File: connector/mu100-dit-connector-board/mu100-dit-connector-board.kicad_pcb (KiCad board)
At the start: 2 copper layers, 37 x 13.9 mm, 8 parts, among them J1 Conn_01x17_Male, J2 Conn_01x17, J3 Conn_01x10_Female

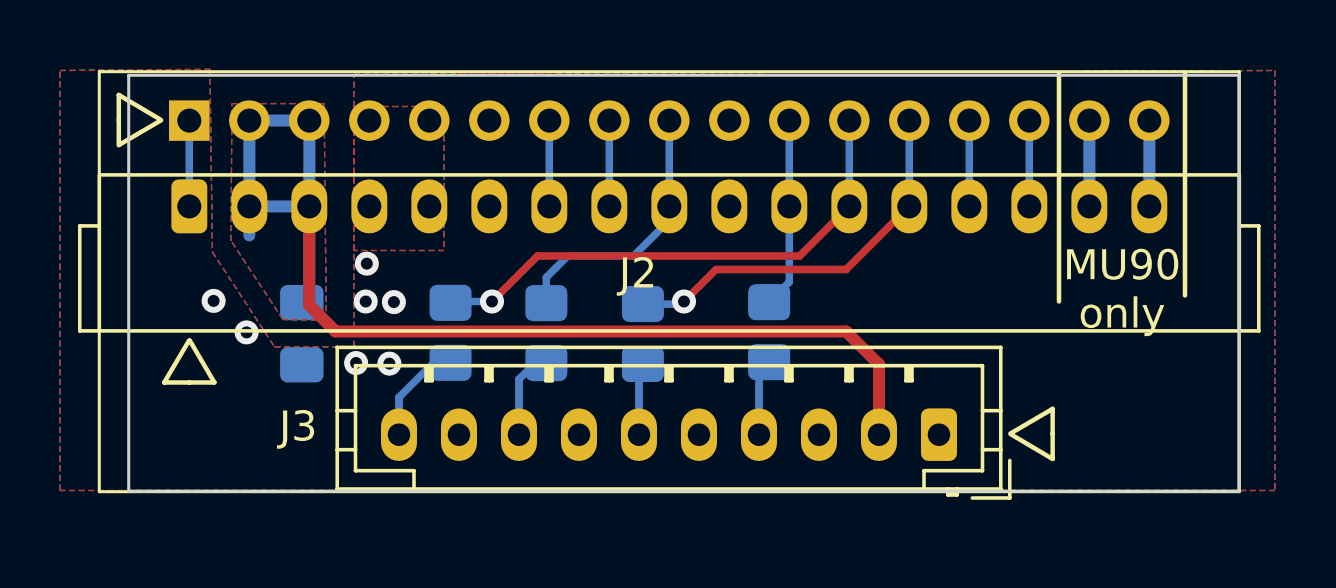
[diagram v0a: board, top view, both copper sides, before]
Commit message: finish connector pcb
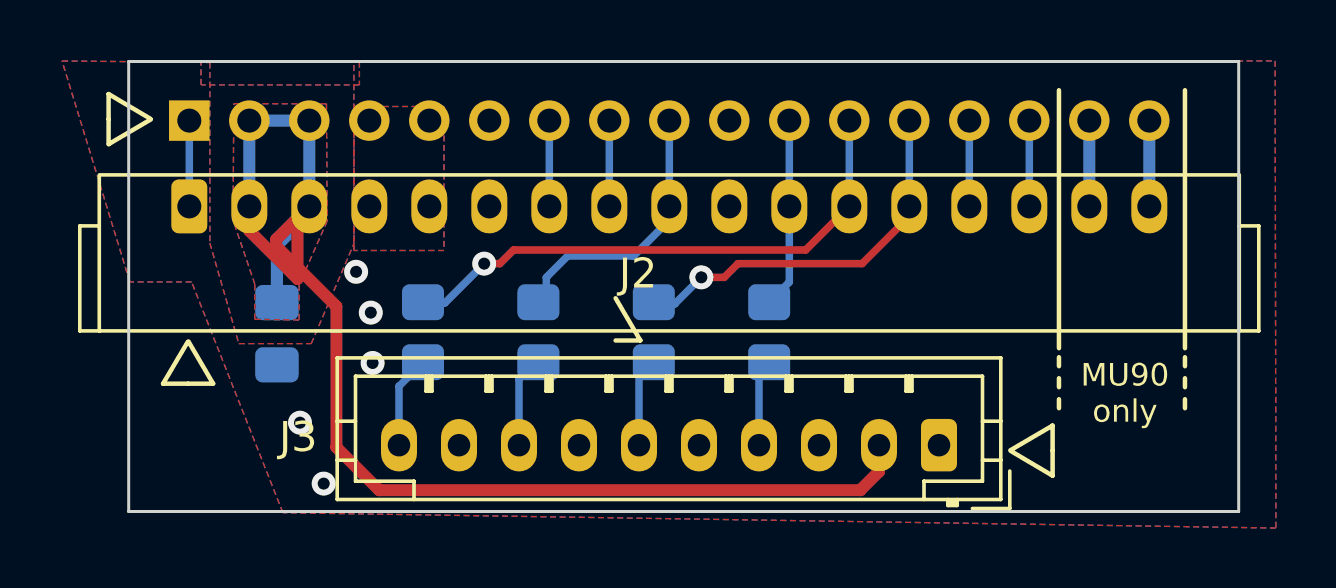
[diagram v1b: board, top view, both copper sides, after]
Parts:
- moved R4 0.92 mm to (73.5, 65.0)
- moved C1 0.83 mm to (68.6, 65.1)
- moved R3 0.37 mm to (81.2, 65.0)
- moved J3 0.35 mm to (90.7, 68.8)
- moved R2 0.27 mm to (77.3, 65.0)
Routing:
- net +5V: track 39.1 -> 49.3 mm
- net /WCLK: track 17.5 -> 18.4 mm
- net /LRCK: track 3.60 -> 2.94 mm
- net GND: track 0.00 -> 0.26 mm, vias 7 -> 5
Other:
- board size 37 x 13.9 mm -> 37 x 15 mm
- board text added: "+9VA"
- board text added: "100"
- board text added: "47"
- board text added: "5V"
- board text added: "AGND"
- board text added: "CK256 (MCLK)"
- board text added: "DACOL (SDAT)"
- board text added: "MELO0"
- board text added: "Molex connector on board"
- board text added: "QCLK (BCK)"
- board text added: "REA"
- board text added: "REB"
- board text added: "RER"
- board text added: "SYOD"
- board text added: "WCLK (LRCK)"
- board text added: "github.com/ nikitalita/ MU100-DIT"

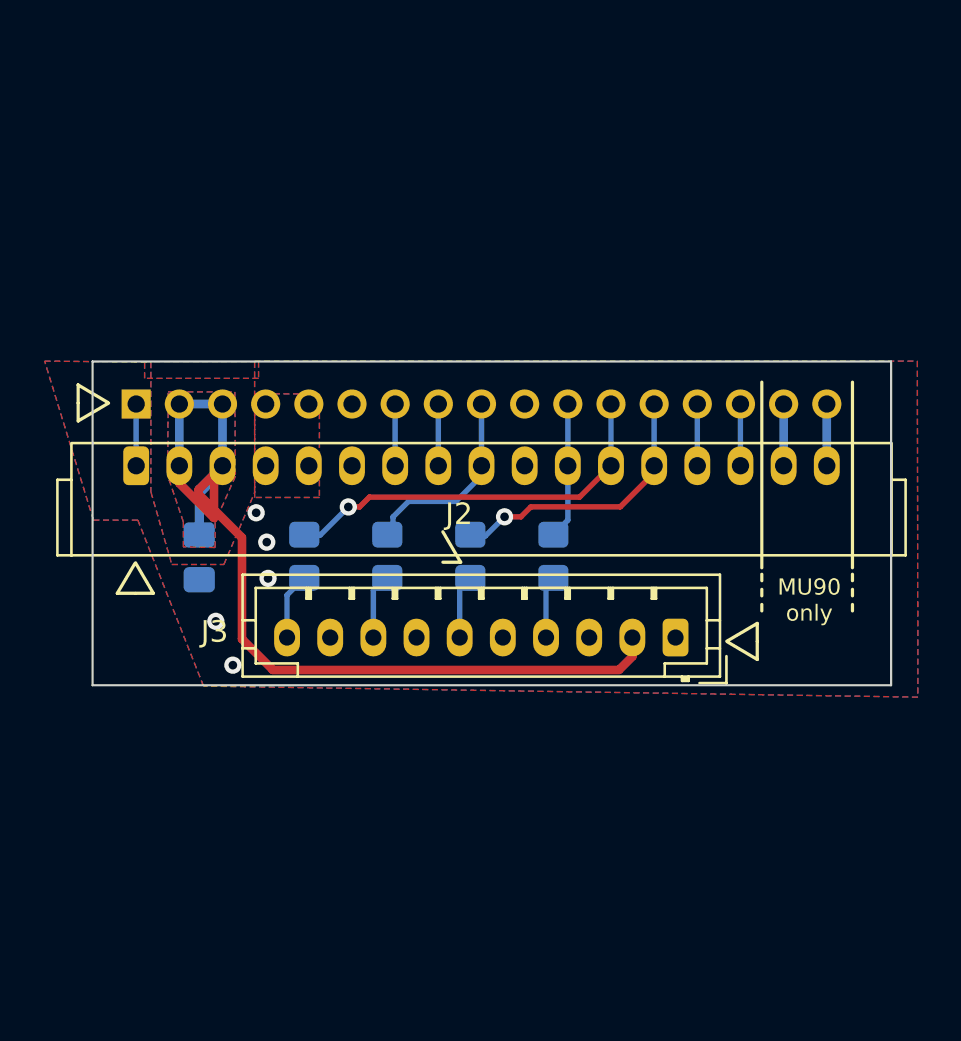
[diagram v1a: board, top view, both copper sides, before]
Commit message: combine pcb projects
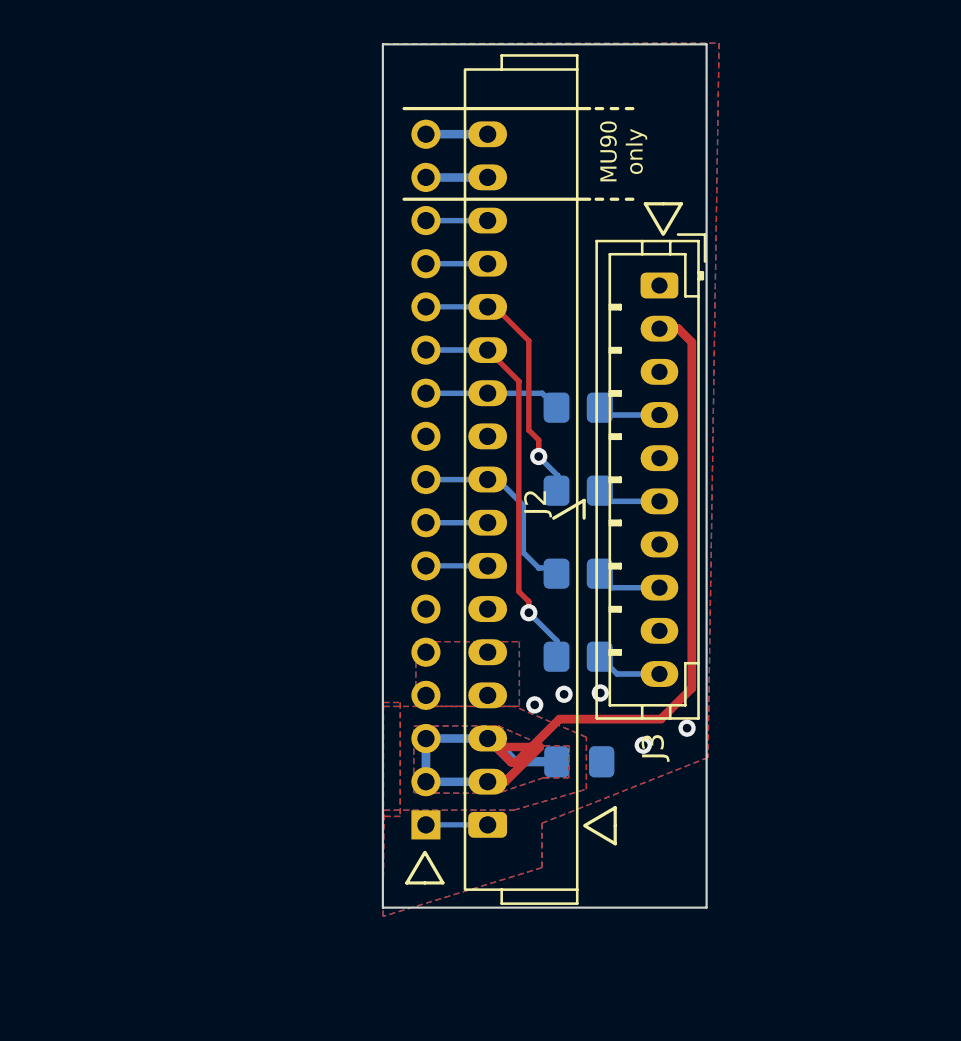
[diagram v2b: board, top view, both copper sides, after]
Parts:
- moved J1 23.7 mm to (79.1, 77.5), turned to 0 degrees
- moved J2 23.3 mm to (82.0, 77.5), turned to 90 degrees
- moved C1 20.0 mm to (86.2, 74.5), turned to 0 degrees
- moved J3 16.3 mm to (90.0, 52.5), turned to -90 degrees
- moved R4 13.5 mm to (86.2, 69.7), turned to 0 degrees
- moved R2 8.88 mm to (86.2, 65.8), turned to 0 degrees
- moved R1 6.98 mm to (86.2, 58.1), turned to 0 degrees
- moved R3 5.85 mm to (86.2, 62.0), turned to 0 degrees
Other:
- board size 37 x 15 mm -> 15 x 40 mm

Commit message: WIP
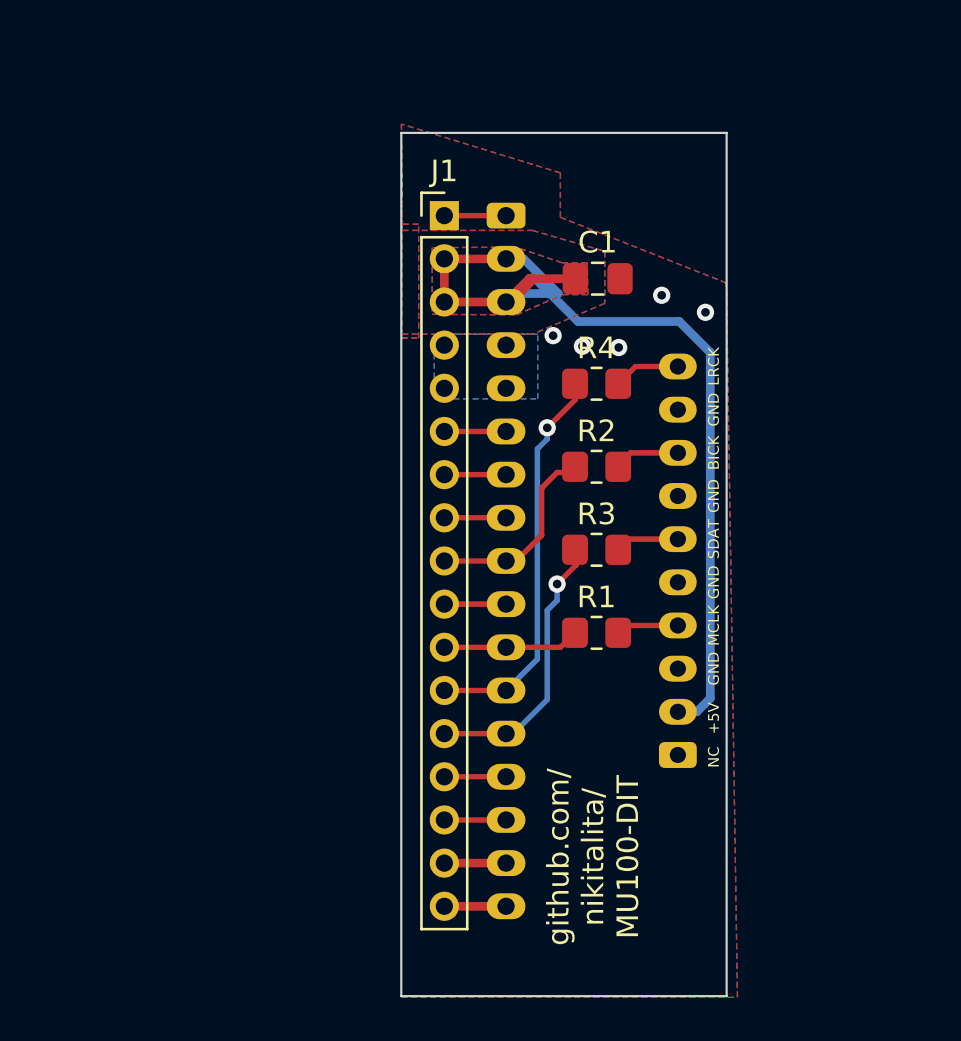
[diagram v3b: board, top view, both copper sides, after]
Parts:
- C1, J1, R1, R2, R3, R4: moved to F.Cu
- J2: value Conn_01x17 -> 51247 Molex; moved to B.Cu
- J3: value Conn_01x10_Female -> JST-PH_01x10_Socket; moved to B.Cu
- moved J1 28.2 mm to (80.0, 49.2)
- moved J2 28.2 mm to (82.8, 49.2), turned to -90 degrees
- moved C1 22.4 mm to (87.1, 52.2)
- moved J3 21.8 mm to (90.8, 74.2), turned to 90 degrees
- moved R4 12.7 mm to (87.0, 57.0)
- moved R1 10.5 mm to (87.0, 68.6)
- moved R2 5.03 mm to (87.0, 60.9)
- moved R3 2.87 mm to (87.0, 64.7)
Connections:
- J1 pad 10: unconnected-(J1-Pad10) -> Net-(J1-Pad10)
- J1 pad 6: unconnected-(J1-Pad6) -> Net-(J1-Pad6)
- J2 pad 10: unconnected-(J2-Pad10) -> Net-(J1-Pad10)
- J2 pad 6: unconnected-(J2-Pad6) -> Net-(J1-Pad6)
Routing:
- net Net-(J1-Pad6): track 0.00 -> 2.86 mm
- net Net-(J1-Pad10): track 0.00 -> 2.86 mm
- net +5V: track 49.3 -> 46.8 mm
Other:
- board size 15 x 40 mm -> 15.1 x 40 mm
- board text added: "16-17 MU90 only"
- board text added: "MU90/100R: Slots into Molex connector MU90/100: Soldered onto unpopulated header"
- board text removed: "MU90 only"
- board text removed: "Molex connector on board"
